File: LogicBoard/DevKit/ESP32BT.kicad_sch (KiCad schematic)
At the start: 16 parts, among them J1 USBC Socket, J15 ESPUartConn, J17 Micro_SD_Card_Det1, U10 ESP32-C3-WROOM-02-N4

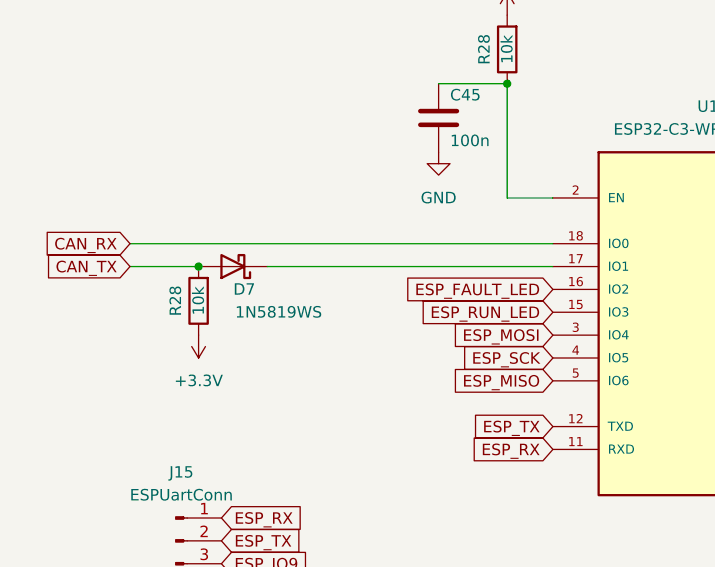
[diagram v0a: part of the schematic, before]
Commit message: initialv2
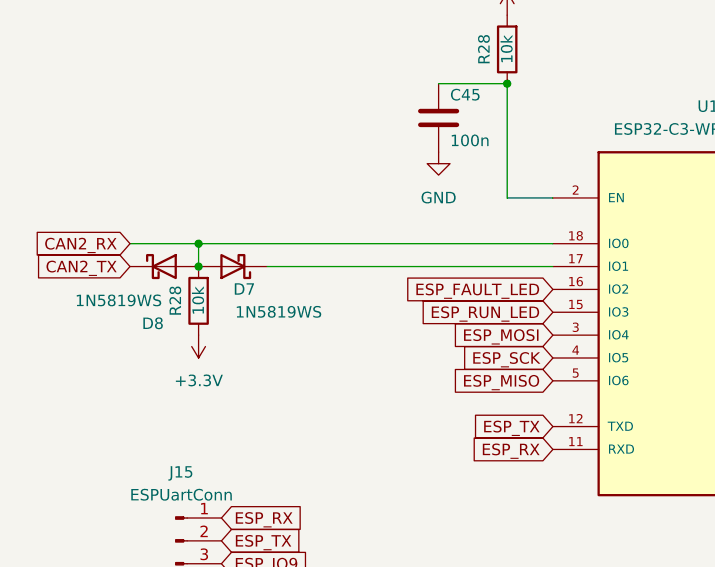
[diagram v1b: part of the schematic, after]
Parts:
- added D8: 1N5819WS, Diode_SMD:D_SOD-323, symbol Device:D_Schottky
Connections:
- net CAN_TX is gone; now on net CAN2_RX: D7.2 (A), R28.2
- net CAN_RX renamed CAN2_RX
- net CAN2_RX: now also D8.2 (A)
- new net CAN2_TX: D8.1 (K)
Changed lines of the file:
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@@
 (kicad_sch (version 20230121) (generator eeschema)
   (paper "A4")
+  (junction (at 73.66 67.31) (diameter 0) (color 0 0 0 0)
+  )
+  (junction (at 73.66 64.77) (diameter 0) (color 0 0 0 0)
+  )
   (junction (at 107.95 46.99) (diameter 0) (color 0 0 0 0)
   )
   (junction (at 199.39 71.12) (diameter 0) (color 0 0 0 0)
-  )
-  (junction (at 73.66 67.31) (diameter 0) (color 0 0 0 0)
   )
   (junction (at 184.15 96.52) (diameter 0) (color 0 0 0 0)
@@
     (stroke (width 0) (type default))
   )
+  (wire (pts (xy 73.66 64.77) (xy 113.03 64.77))
+    (stroke (width 0) (type default))
+  )
   (wire (pts (xy 205.74 64.77) (xy 205.74 49.53))
     (stroke (width 0) (type default))
@@
     (stroke (width 0) (type default))
   )
-  (wire (pts (xy 66.04 67.31) (xy 73.66 67.31))
-    (stroke (width 0) (type default))
-  )
-  (wire (pts (xy 66.04 64.77) (xy 113.03 64.77))
+  (wire (pts (xy 66.04 64.77) (xy 73.66 64.77))
     (stroke (width 0) (type default))
   )
@@
   )
   (wire (pts (xy 199.39 69.85) (xy 199.39 71.12))
+    (stroke (width 0) (type default))
+  )
+  (wire (pts (xy 73.66 64.77) (xy 73.66 67.31))
     (stroke (width 0) (type default))
   )
@@
     (effects (font (size 3.27 3.27)) (justify left bottom))
   )
-  (global_label "CAN_TX" (shape input) (at 66.04 67.31 180) (fields_autoplaced)
-    (effects (font (size 1.27 1.27)) (justify right))
-    (property "Intersheetrefs" "${INTERSHEET_REFS}" (at 56.9546 67.31 0)
-      (effects (font (size 1.27 1.27)) (justify right) hide)
-    )
-  )
   (global_label "ESP_FAULT_LED" (shape input) (at 158.75 138.43 180) (fields_autoplaced)
     (effects (font (size 1.27 1.27)) (justify right))
@@
     )
   )
-  (global_label "CAN_RX" (shape input) (at 66.04 64.77 180) (fields_autoplaced)
-    (effects (font (size 1.27 1.27)) (justify right))
-    (property "Intersheetrefs" "${INTERSHEET_REFS}" (at 56.6522 64.77 0)
+  (global_label "CAN2_TX" (shape input) (at 66.04 67.31 180) (fields_autoplaced)
+    (effects (font (size 1.27 1.27)) (justify right))
+    (property "Intersheetrefs" "${INTERSHEET_REFS}" (at 55.7451 67.31 0)
       (effects (font (size 1.27 1.27)) (justify right) hide)
     )
@@
     (property "Intersheetrefs" "${INTERSHEET_REFS}" (at 158.5825 69.85 0)
       (effects (font (size 1.27 1.27)) (justify left) hide)
+    )
+  )
+  (global_label "CAN2_RX" (shape input) (at 66.04 64.77 180) (fields_autoplaced)
+    (effects (font (size 1.27 1.27)) (justify right))
+    (property "Intersheetrefs" "${INTERSHEET_REFS}" (at 55.4427 64.77 0)
+      (effects (font (size 1.27 1.27)) (justify right) hide)
     )
   )
@@
         )
       )
+    )
+  )
+  (symbol (lib_id "Device:D_Schottky") (at 69.85 67.31 0) (unit 1)
+    (in_bom yes) (on_board yes) (dnp no)
+    (property "Reference" "D8" (at 68.58 73.66 0)
+      (effects (font (size 1.27 1.27)))
+    )
+    (property "Value" "1N5819WS" (at 64.77 71.12 0)
+      (effects (font (size 1.27 1.27)))
+    )
+    (property "Footprint" "Diode_SMD:D_SOD-323" (at 69.85 67.31 0)
+      (effects (font (size 1.27 1.27)) hide)
+    )
+    (property "Datasheet" "~" (at 69.85 67.31 0)
+      (effects (font (size 1.27 1.27)) hide)
+    )
+    (property "MPN" "C191023" (at 69.85 67.31 0)
+      (effects (font (size 1.27 1.27)) hide)
+    )
+    (pin "1")
+    (pin "2")
+    (instances
+      (project "DevKit"
+        (path "/768a484b-8a27-40cf-8cad-0f63935b1af0/72793ee1-8b24-4ded-a030-5a38e70b572c"
+          (reference "D8") (unit 1)
+        )
+      )
